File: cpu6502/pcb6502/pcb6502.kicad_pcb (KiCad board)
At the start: 2 copper layers, 111.8 x 109.2 mm, 34 parts, among them J1 Power, J2 RS232, J3 VIA PA, J4 VIA PB, J5 Ext RST, SW1 Reset, U1 6502, U2 EEPROM, U3 RAM, U4 65C22, U5 74HC00, U6 L7805, U7 W65C51NxP, U8 MAX232, X1 1MHz, Y1 Crystal

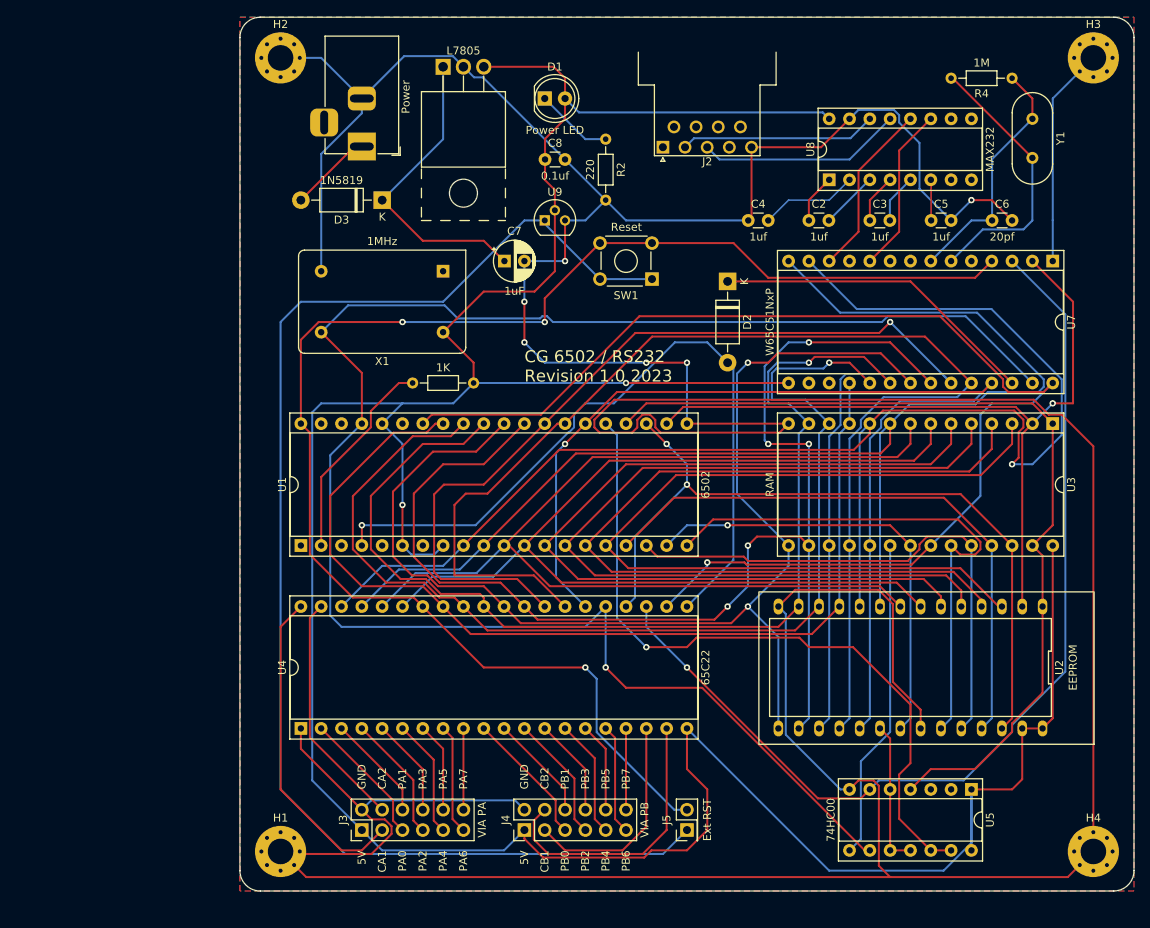
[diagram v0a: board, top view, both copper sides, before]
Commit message: Finished the PCB
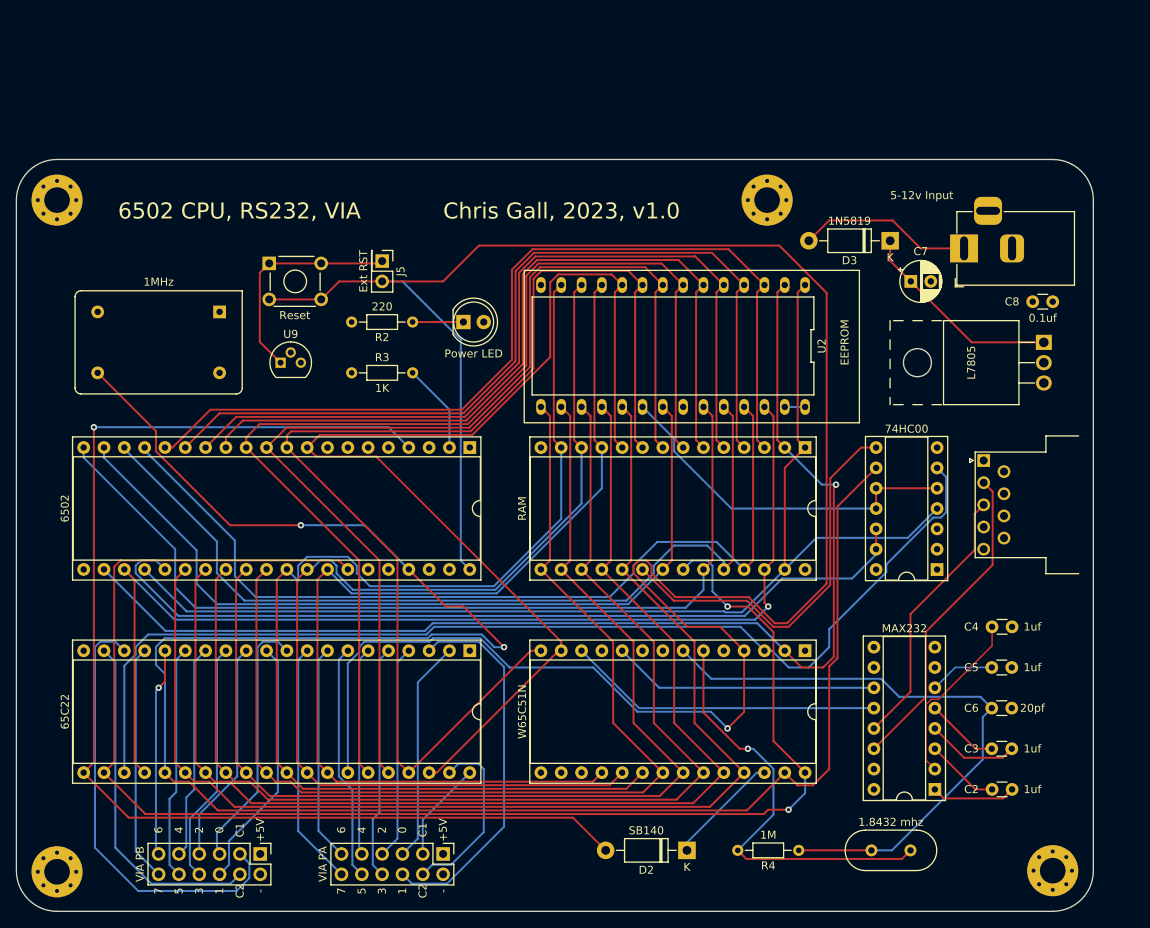
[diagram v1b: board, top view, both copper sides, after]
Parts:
- removed Y1: Crystal, Crystal:Crystal_HC49-4H_Vertical
- added 1.8432 mhz: Crystal, Crystal:Crystal_HC49-4H_Vertical, F.Cu at (157.7, 132.1)
- C6: value 20pf -> 20pf
- U7: value W65C51NxP -> W65C51N
- moved H3 164.7 mm to (55.9, 134.8)
- moved H1 101.6 mm to (144.6, 50.8)
- moved R4 100.1 mm to (148.6, 132.1)
- moved U6 82.6 mm to (179.2, 68.6), turned to -90 degrees
- moved J5 80.7 mm to (96.5, 58.4), turned to -90 degrees
- moved U8 77.3 mm to (165.6, 124.5), turned to 180 degrees
- moved J1 76.3 mm to (169.3, 56.8), turned to 180 degrees
- moved C2 75.5 mm to (175.3, 124.5), turned to 180 degrees
- moved D2 71.3 mm to (134.6, 132.1), turned to 180 degrees
- moved C3 68.4 mm to (175.2, 119.4), turned to 180 degrees
- moved D3 63.7 mm to (160.0, 55.9)
- moved C8 63.5 mm to (177.8, 63.5)
- moved C6 61.0 mm to (172.7, 114.3)
- moved C4 60.6 mm to (175.3, 104.1), turned to 180 degrees
- moved U7 57.7 mm to (149.4, 107.1)
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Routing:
- net GND: track 627.5 -> 0.00 mm, vias 6 -> 0
- net +5V: track 397.7 -> 2.54 mm, vias 2 -> 0
- net Net-(J5-Pin_1): track 168.8 -> 28.2 mm
- net /RST: track 187.3 -> 280.4 mm, vias 3 -> 1
- net /IRQ: track 92.9 -> 153.4 mm
- net /A12: track 96.9 -> 148.7 mm
- net /A10: track 56.0 -> 104.2 mm, vias 1 -> 0
- net /A11: track 67.9 -> 114.1 mm
- net /XTAL2: track 30.7 -> 76.1 mm
- net /A9: track 66.9 -> 111.7 mm
- net /A13: track 95.3 -> 136.3 mm, vias 2 -> 1
- net /A8: track 74.1 -> 111.6 mm
- net /A0: track 178.6 -> 141.2 mm, vias 1 -> 0
- net /PHI2: track 220.5 -> 256.0 mm, vias 1 -> 2
- net /PA1: track 13.3 -> 47.2 mm
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- added copper zone on In2.Cu, net +5V
- added copper zone on In1.Cu, net GND
- removed copper zone on B.Cu, net GND
- removed copper zone on F.Cu, net GND
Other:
- board size 111.8 x 109.2 mm -> 134.6 x 94 mm
- copper layers 2 -> 4
- board text added: "+5V"
- board text added: "-"
- board text added: "0"
- board text added: "1"
- board text added: "2"
- board text added: "3"
- board text added: "4"
- board text added: "5"
- board text added: "5-12v Input"
- board text added: "6"
- board text added: "6502 CPU, RS232, VIA"
- board text added: "7"
- board text added: "C1"
- board text added: "C2"
- board text added: "Chris Gall, 2023, v1.0"
- board text removed: "5V"
- board text removed: "CA1"
- board text removed: "CA2"
- board text removed: "CB1"
- board text removed: "CB2"
- board text removed: "CG 6502 / RS232 Revision 1.0 2023"
- board text removed: "GND"
- board text removed: "PA0"
- board text removed: "PA1"
- board text removed: "PA2"
- board text removed: "PA3"
- board text removed: "PA4"
- board text removed: "PA5"
- board text removed: "PA6"
- board text removed: "PA7"
- board text removed: "PB0"
- board text removed: "PB1"
- board text removed: "PB2"
- board text removed: "PB3"
- board text removed: "PB4"
- board text removed: "PB5"
- board text removed: "PB6"
- board text removed: "PB7"
